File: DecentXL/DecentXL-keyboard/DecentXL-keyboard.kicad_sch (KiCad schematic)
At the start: 212 parts, among them J1 Conn_02x12_Odd_Even, J2 Conn_01x26, J3 Conn_01x04, J4 Conn_01x10, J5 Conn_01x10, J6 Conn_01x10, J7 Conn_01x10, SW0 SW_Push_45deg, SW1 SW_Push_45deg, SW2 SW_Push_45deg, SW3 SW_Push_45deg, SW4 SW_Push_45deg, SW5 SW_Push_45deg, SW6 SW_Push_45deg, SW8 SW_Push_45deg, SW9 SW_Push_45deg

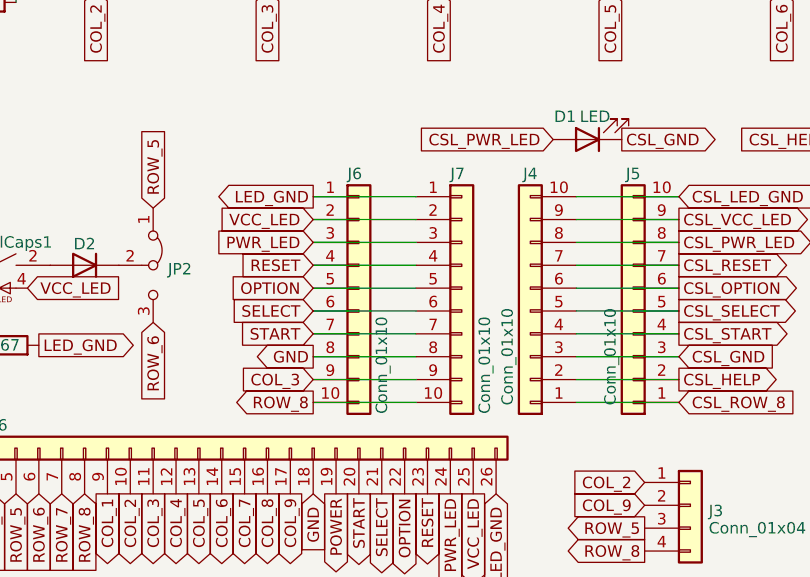
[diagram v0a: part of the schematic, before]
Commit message: DecentXL rev 1
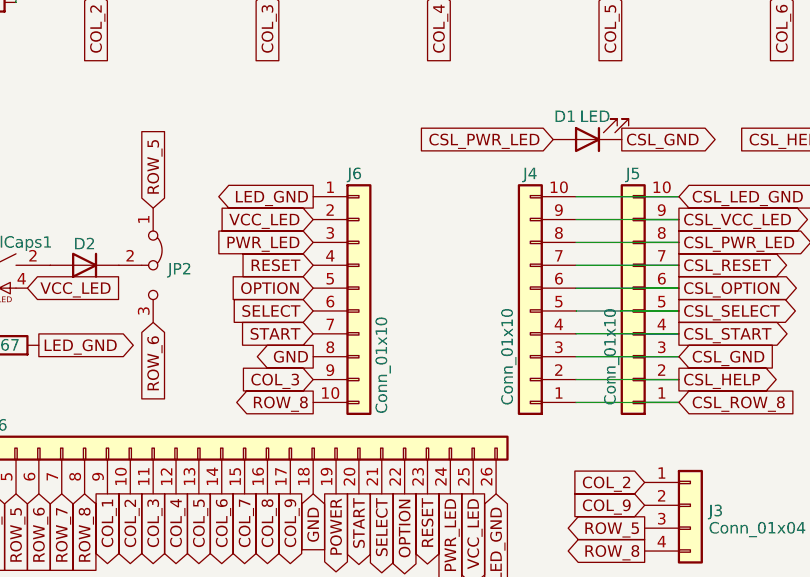
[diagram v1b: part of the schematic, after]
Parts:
- removed J7: Conn_01x10, Connector_PinHeader_2.54mm:PinHeader_1x10_P2.54mm_Vertical, symbol Connector_Generic:Conn_01x10
- D1: JLC Part (none) -> C2290
- D100, D101, D102, D103, D104, D105, D106, D107, D108, D109, D110, D111, D112, D113, D114, D115, D116, D117, D118, D119, D120, D121, D122, D123, D124, D125, D126, D127, D128, D2, D69, D70, D71, D72, D73, D74, D75, D76, D77, D78, D79, D80, D81, D82, D83, D84, D85, D86, D87, D88, D89, D90, D91, D92, D93, D94, D95, D96, D97, D98, D99: JLC Part (none) -> C81598
- J1, J3, J4, RV1: now left out of the parts list
- J2: JLC Part (none) -> C60248
- J5, J6: footprint Connector_FFC-FPC:TE_1-1734839-0_1x10-1MP_P0.5mm_Horizontal -> Connector_FFC-FPC:Hirose_FH12-10S-0.5SH_1x10-1MP_P0.50mm_Horizontal; JLC Part (none) -> C709365
- R10, R11, R12, R13, R14, R15, R16, R17, R18, R19, R2, R20, R21, R22, R23, R24, R25, R26, R27, R28, R29, R3, R30, R31, R32, R33, R34, R35, R36, R37, R38, R39, R4, R40, R41, R42, R43, R44, R45, R46, R47, R48, R49, R5, R50, R51, R52, R53, R54, R55, R56, R57, R58, R59, R6, R61, R62, R63, R64, R65, R66, R67, R7, R8, R9: JLC Part (none) -> C22775
- SW0, SW1, SW2, SW3, SW4, SW5, SW6, SW8, SW9, SWA1, SWB1, SWBrk1, SWBrk2, SWC1, SWComma1, SWCps1, SWCtl1, SWCtlCaps1, SWD1, SWDash1, SWDel1, SWDel2, SWE1, SWEqual1, SWEsc1, SWF1, SWFn1, SWFn2, SWFn3, SWFn4, SWG1, SWGT1, SWH1, SWHlp1, SWI1, SWInv1, SWJ1, SWK1, SWL1, SWLT1, SWLeftSft1, SWM1, SWN1, SWO1, SWOption1, SWP1, SWPeriod1, SWPlus1, SWQ1, SWR1, SWReset1, SWRet1, SWRet2, SWRightSft1, SWS1, SWSelect1, SWSemi1, SWSlash1, SWSpc1, SWStar1, SWStart1, SWT1, SWTab1, SWU1, SWV1, SWW1, SWX1, SWY1, SWZ1: JLC Part (none) -> C193191
